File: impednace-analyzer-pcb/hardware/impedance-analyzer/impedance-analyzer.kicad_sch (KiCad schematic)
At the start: 8 parts, among them U1 AD9833BRMZ, Y1 ABM3-25.000MHZ-J2Y-T

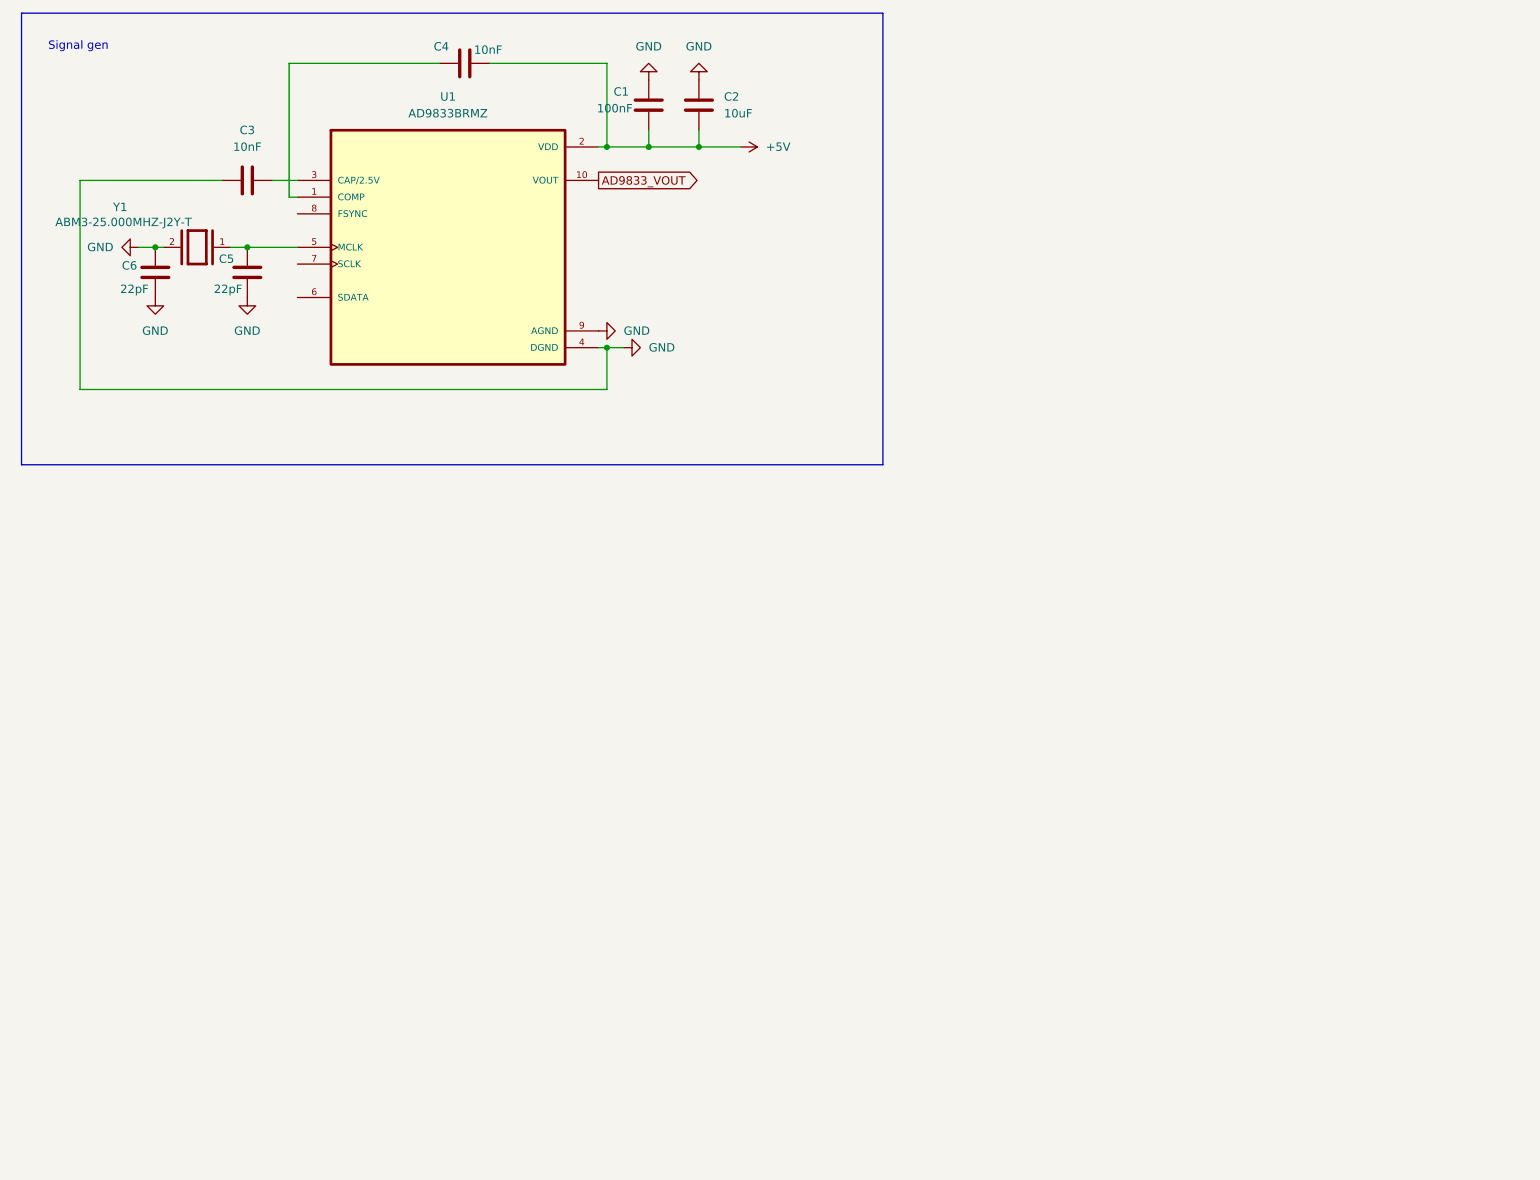
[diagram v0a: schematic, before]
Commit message: did schematic work
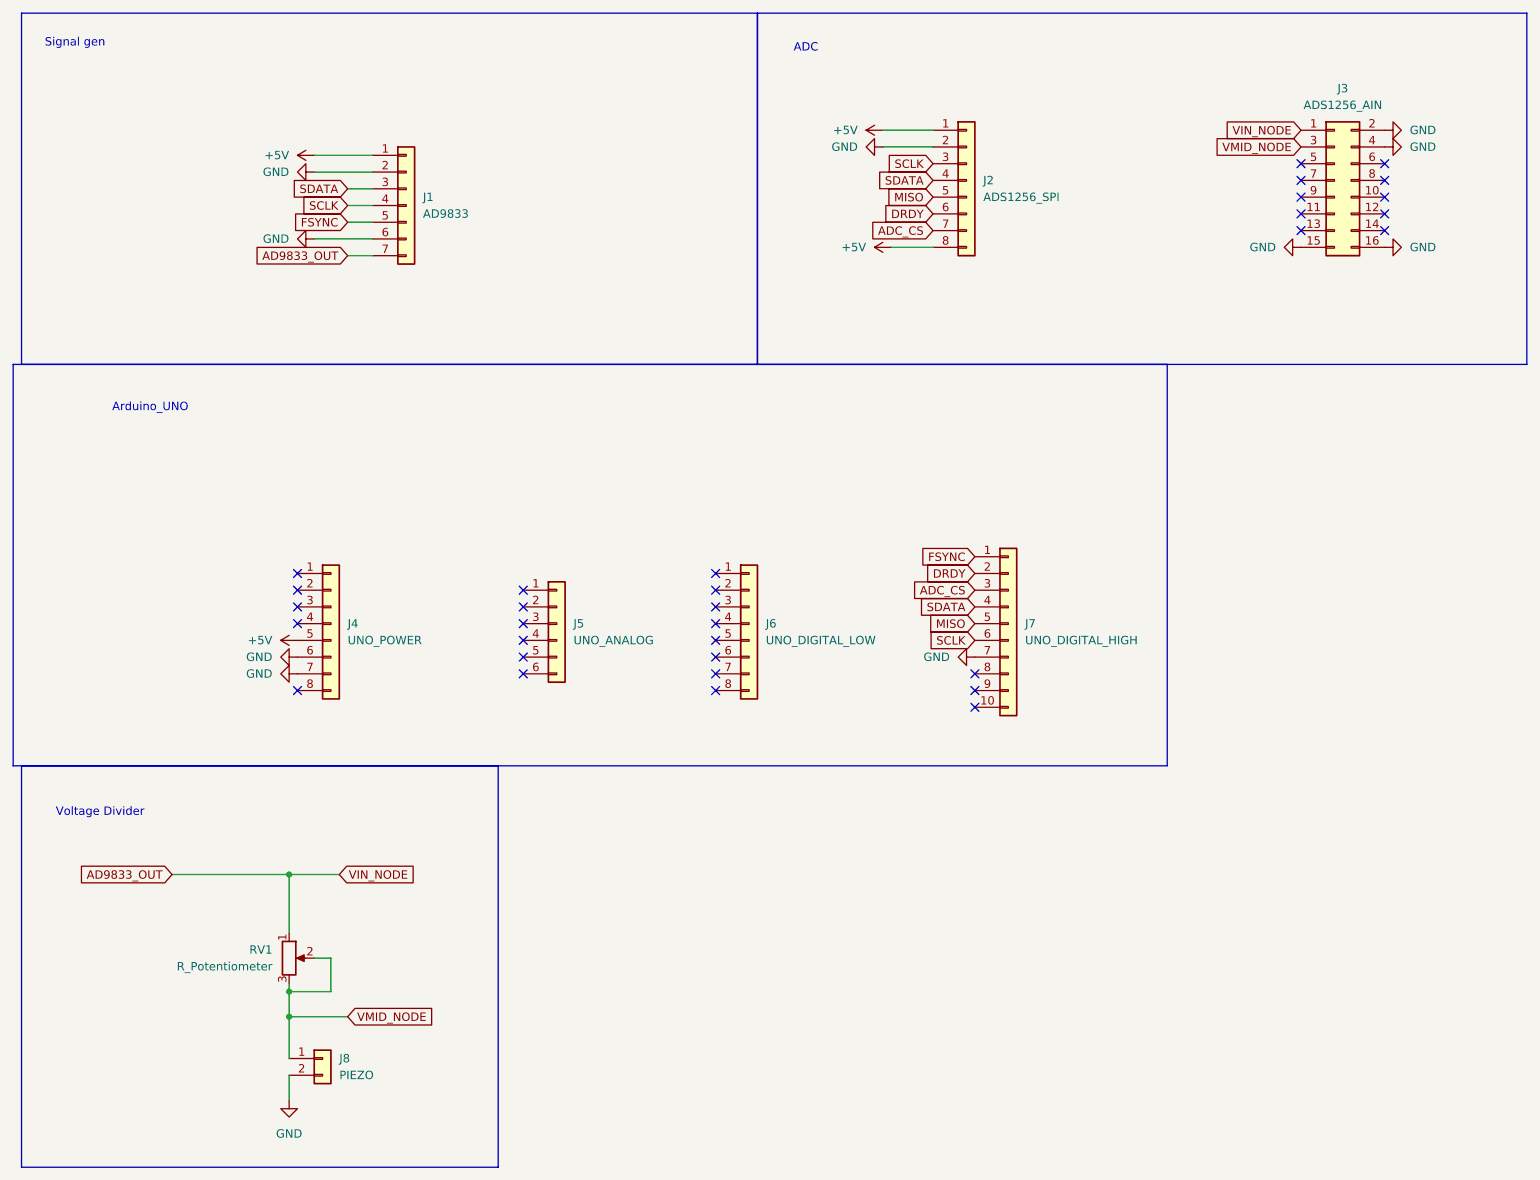
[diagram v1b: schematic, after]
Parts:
- removed C1: 100nF, symbol Device:C
- removed C2: 10uF, symbol Device:C
- removed C3, C4: 10nF, symbol Device:C
- removed C5, C6: 22pF, symbol Device:C
- removed U1: AD9833BRMZ, impedance-analyzer:SOP50P490X110-10N, symbol ImpedanceAnalyzer:AD9833BRMZ
- removed Y1: ABM3-25.000MHZ-J2Y-T, ABM3-25.000MHZ-J2Y-T:XTAL_ABM3-25.000MHZ-J2Y-T, symbol ImpedanceAnalyzer:ABM3-25.000MHZ-J2Y-T
- added J1: AD9833, symbol Connector_Generic:Conn_01x07
- added J2: ADS1256_SPI, symbol Connector_Generic:Conn_01x08
- added J3: ADS1256_AIN, symbol Connector_Generic:Conn_02x08_Odd_Even
- added J4: UNO_POWER, symbol Connector_Generic:Conn_01x08
- added J5: UNO_ANALOG, symbol Connector_Generic:Conn_01x06
- added J6: UNO_DIGITAL_LOW, symbol Connector_Generic:Conn_01x08
- added J7: UNO_DIGITAL_HIGH, symbol Connector_Generic:Conn_01x10
- added J8: PIEZO, symbol Connector_Generic:Conn_01x02
- added RV1: R_Potentiometer, symbol Device:R_Potentiometer
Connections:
- net +5V: now also J1.1 (Pin_1), J2.1 (Pin_1), J2.8 (Pin_8), J4.5 (Pin_5)
- net GND: now also J1.2 (Pin_2), J1.6 (Pin_6), J2.2 (Pin_2), J3.15 (Pin_15), J3.16 (Pin_16), J3.2 (Pin_2), J3.4 (Pin_4), J4.6 (Pin_6), J4.7 (Pin_7), J7.7 (Pin_7), J8.2 (Pin_2)
- new net AD9833_OUT: J1.7 (Pin_7), J3.1 (Pin_1), RV1.1
- new net ADC_CS: J2.7 (Pin_7), J7.3 (Pin_3)
- new net DRDY: J2.6 (Pin_6), J7.2 (Pin_2)
- new net FSYNC: J1.5 (Pin_5), J7.1 (Pin_1)
- new net MISO: J2.5 (Pin_5), J7.5 (Pin_5)
- new net SCLK: J1.4 (Pin_4), J2.3 (Pin_3), J7.6 (Pin_6)
- new net SDATA: J1.3 (Pin_3), J2.4 (Pin_4), J7.4 (Pin_4)
- new net VMID_NODE: J3.3 (Pin_3), J8.1 (Pin_1), RV1.2, RV1.3
- no-connect marks 0 -> 32
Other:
- note added: "ADC"
- note added: "Arduino_UNO"
- note added: "Voltage Divider"
